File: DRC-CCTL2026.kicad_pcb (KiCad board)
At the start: 2 copper layers, 80 x 60 mm, 72 parts, among them J1 USB, J10 SW3, J12 LCD_BackLight, J2 FDCAN1, J3 FDCAN2, J4 FDCAN3, J5 SW1, J6 SW2, J7 STLINK, J8 I2C, J9 USART, Q1 MMBT3904, SW1 RESET, SW2 DIP, U1 STM32G474RETx, U2 AZ1084C-3.3, U3 74AHC1G125, Y1 8M10PB/XT324-10/80

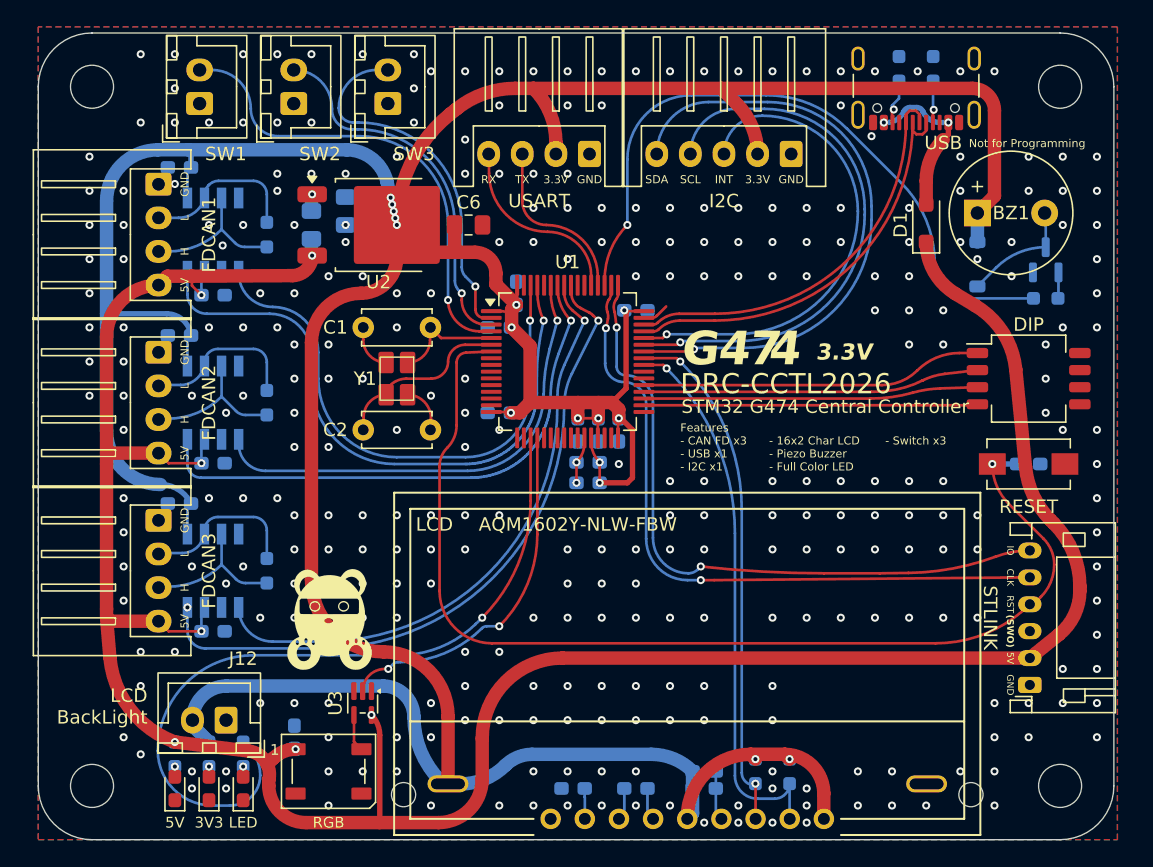
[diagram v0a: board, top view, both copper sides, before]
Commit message: v0.2.0
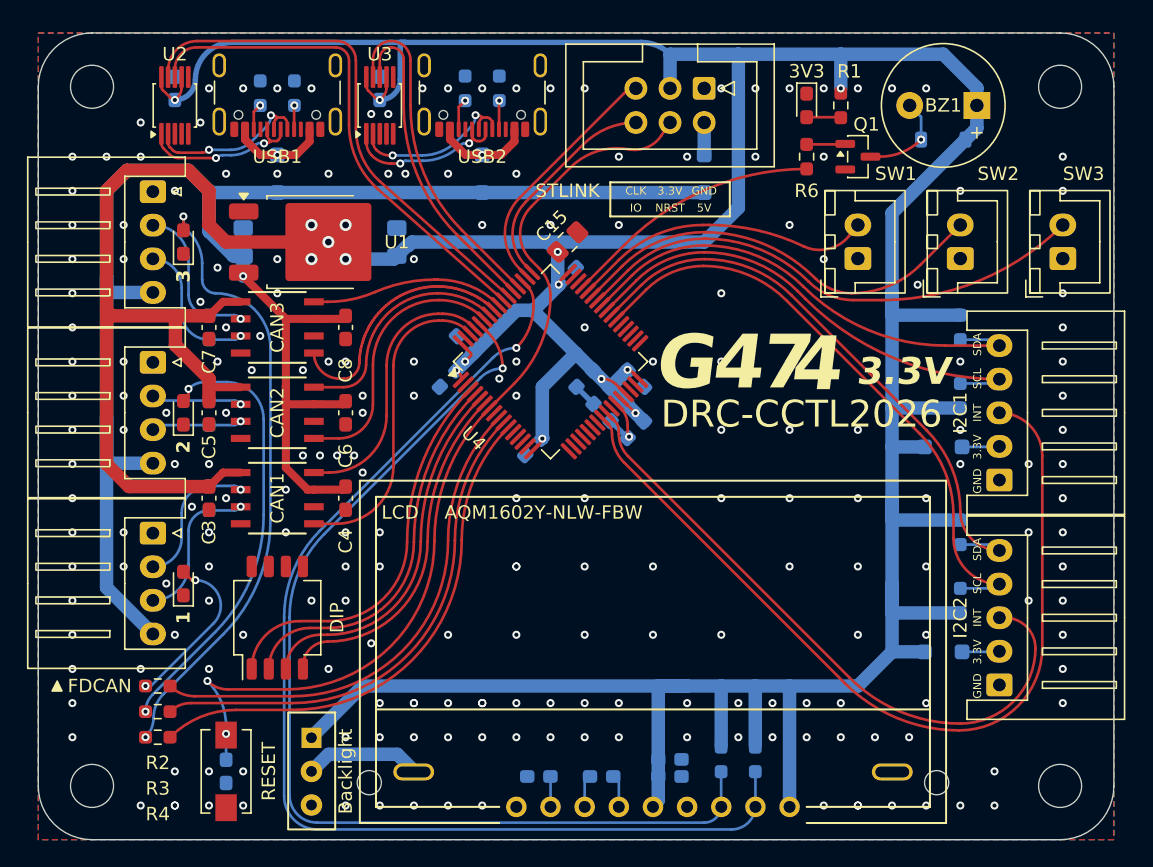
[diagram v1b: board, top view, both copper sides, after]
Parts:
- removed the C1 at (139.2, 91.9)
- removed the C10 at (145.6, 89.4)
- removed the C11 at (150.1, 99.5)
- removed the C12 at (151.7, 99.5)
- removed the C2 at (134.2, 99.5)
- removed the C3 at (183.7, 102.1)
- removed the C6 at (142.0, 84.3)
- removed the C7 at (144.3, 98.2)
- removed the C8 at (153.2, 99.5)
- removed the C9 at (154.4, 90.6)
- removed the D1 at (176.0, 84.2)
- removed the J1 at (175.3, 73.0)
- removed J12: LCD_BackLight, Connector_JST:JST_XH_B2B-XH-A_1x02_P2.50mm_Vertical
- removed the R1 at (176.6, 72.7)
- removed R5: 1k, Resistor_SMD:R_0603_1608Metric_Pad0.98x0.95mm_HandSolder
- removed the R6 at (125.2, 123.7)
- removed the SW1 at (183.7, 102.1)
- removed the U1 at (149.4, 94.4)
- removed Y1: 8M10PB/XT324-10/80, lib:8M10PB_XT324-10_80
- added C17: 0.1u, Capacitor_SMD:C_0603_1608Metric_Pad1.08x0.95mm_HandSolder, B.Cu at (154.4, 95.7)
- added C18: 0.1u, Capacitor_SMD:C_0603_1608Metric_Pad1.08x0.95mm_HandSolder, B.Cu at (149.4, 88.1)
- added C19: 0.1u, Capacitor_SMD:C_0603_1608Metric_Pad1.08x0.95mm_HandSolder, B.Cu at (141.8, 93.2)
- added C20: 1u, Capacitor_SMD:C_0603_1608Metric_Pad1.08x0.95mm_HandSolder, B.Cu at (150.6, 95.7)
- added C21: 0.1u, Capacitor_SMD:C_0603_1608Metric_Pad1.08x0.95mm_HandSolder, B.Cu at (151.9, 97.0)
- added C22: 1u, Capacitor_SMD:C_0603_1608Metric_Pad1.08x0.95mm_HandSolder, B.Cu at (154.4, 99.5)
- added C23: 0.1u, Capacitor_SMD:C_0603_1608Metric_Pad1.08x0.95mm_HandSolder, B.Cu at (153.2, 98.2)
- added C24: 1u, Capacitor_SMD:C_0603_1608Metric_Pad1.08x0.95mm_HandSolder, B.Cu at (140.5, 95.7)
- added C25: 0.1u, Capacitor_SMD:C_0603_1608Metric_Pad1.08x0.95mm_HandSolder, B.Cu at (124.0, 124.9)
- added D10: SS2040FL, Diode_SMD:D_SOD-123F, B.Cu at (127.8, 80.5)
- added D11: SS2040FL, Diode_SMD:D_SOD-123F, B.Cu at (143.0, 80.5)
- added D3: SS2040FL, Diode_SMD:D_SOD-123F, B.Cu at (177.3, 100.8)
- added D7: LED2, LED_SMD:LED_0603_1608Metric_Pad1.05x0.95mm_HandSolder, F.Cu at (120.8, 98.2)
- added D8: LED3, LED_SMD:LED_0603_1608Metric_Pad1.05x0.95mm_HandSolder, F.Cu at (120.8, 85.5)
- added J10: USB_C, Connector_USB:USB_C_Receptacle_GCT_USB4105-xx-A_16P_TopMnt_Horizontal, F.Cu at (127.8, 73.5)
- added J11: USB_C, Connector_USB:USB_C_Receptacle_GCT_USB4105-xx-A_16P_TopMnt_Horizontal, F.Cu at (143.0, 73.5)
- added R12: 5.1k, Resistor_SMD:R_0603_1608Metric_Pad0.98x0.95mm_HandSolder, B.Cu at (129.1, 74.5)
- added R13: 5.1k, Resistor_SMD:R_0603_1608Metric_Pad0.98x0.95mm_HandSolder, B.Cu at (126.5, 74.5)
- added R14: 5.1k, Resistor_SMD:R_0603_1608Metric_Pad0.98x0.95mm_HandSolder, B.Cu at (144.3, 74.1)
- added R15: 5.1k, Resistor_SMD:R_0603_1608Metric_Pad0.98x0.95mm_HandSolder, B.Cu at (141.8, 74.1)
- added R16: 4.7k, Resistor_SMD:R_0603_1608Metric_Pad0.98x0.95mm_HandSolder, B.Cu at (178.6, 91.9)
- added R17: 4.7k, Resistor_SMD:R_0603_1608Metric_Pad0.98x0.95mm_HandSolder, B.Cu at (178.6, 97.0)
- added R18: 4.7k, Resistor_SMD:R_0603_1608Metric_Pad0.98x0.95mm_HandSolder, B.Cu at (178.6, 107.1)
- added R19: 4.7k, Resistor_SMD:R_0603_1608Metric_Pad0.98x0.95mm_HandSolder, B.Cu at (178.6, 112.2)
- added R3: 1k, Resistor_SMD:R_0603_1608Metric_Pad0.98x0.95mm_HandSolder, F.Cu at (118.9, 120.5)
- added R4: 1k, Resistor_SMD:R_0603_1608Metric_Pad0.98x0.95mm_HandSolder, F.Cu at (118.9, 122.4)
- added SW2: SS-12D00G3, lib:SS-12D00G3, F.Cu at (130.3, 124.9)
- added SW3: SW_Push, Button_Switch_SMD:SW_SPST_EVQPE1, F.Cu at (124.0, 124.9)
- added U2: CH340E, Package_SO:MSOP-10_3x3mm_P0.5mm, F.Cu at (120.2, 75.4)
- added U4: STM32G474RETx, Package_QFP:LQFP-64_10x10mm_P0.5mm, F.Cu at (148.1, 94.4)
- C13, C16: value 1u -> 0.1u
- C15: value 0.1u -> 4.7u; footprint Capacitor_SMD:C_0603_1608Metric_Pad1.08x0.95mm_HandSolder -> Capacitor_SMD:C_0805_2012Metric_Pad1.18x1.45mm_HandSolder; moved to F.Cu
- C3: renamed from C17; moved to F.Cu
- C4: renamed from C18; moved to F.Cu
- C5: renamed from C19; moved to F.Cu
- C6: renamed from C20; moved to F.Cu
- C7: renamed from C21; moved to F.Cu
- C8: renamed from C22; moved to F.Cu
- CAN1: renamed from FDCAN1; footprint footprints:SOIC127P600X175-8N -> lib:SO8_SOT96-1_NXP; moved to F.Cu
- CAN2: renamed from FDCAN2; footprint footprints:SOIC127P600X175-8N -> lib:SO8_SOT96-1_NXP; moved to F.Cu
- CAN3: renamed from FDCAN3; footprint footprints:SOIC127P600X175-8N -> lib:SO8_SOT96-1_NXP; moved to F.Cu
- D2: value 1N4148W -> SS2040FL; footprint Diode_SMD:D_SOD-123 -> Diode_SMD:D_SOD-123F
- D4: value RGB -> SS2040FL; footprint LED_SMD:LED_WS2812B_PLCC4_5.0x5.0mm_P3.2mm -> Diode_SMD:D_SOD-123F; moved to B.Cu
- D5: value 5V -> 1N4148W; footprint LED_SMD:LED_0603_1608Metric_Pad1.05x0.95mm_HandSolder -> Diode_SMD:D_SOD-123; moved to B.Cu
- D6: value LED -> LED1
- G***: moved to B.Cu
- J1: renamed from J7; footprint Connector_JST:JST_PH_S6B-PH-K_1x06_P2.00mm_Horizontal -> Connector_IDC:IDC-Header_2x03_P2.54mm_Vertical
- J8: value I2C -> I2C1
- J9: value USART -> I2C2; footprint Connector_JST:JST_XH_S4B-XH-A_1x04_P2.50mm_Horizontal -> Connector_JST:JST_XH_S5B-XH-A_1x05_P2.50mm_Horizontal
- Q1: moved to F.Cu
- R1: renamed from R4; value 470 -> 1k; moved to F.Cu
- R2: value 5.1k -> 1k; moved to F.Cu
- R6: renamed from R3; moved to F.Cu
- U3: value 74AHC1G125 -> CH340E; footprint Package_TO_SOT_SMD:SOT-353_SC-70-5 -> Package_SO:MSOP-10_3x3mm_P0.5mm
- moved D5 74.8 mm to (177.3, 77.9), turned to 180 degrees
- moved R2 71.7 mm to (118.9, 118.6), turned to 180 degrees
- moved D1 67.5 mm to (167.2, 75.4), turned to -90 degrees
- moved R1 67.4 mm to (169.7, 75.4)
- moved SW1 58.6 mm to (127.8, 113.5), turned to 90 degrees
- moved J7 51.5 mm to (186.2, 86.8)
- moved J6 50.9 mm to (178.6, 86.8)
- moved J1 50.6 mm to (159.5, 74.1), turned to -90 degrees
- moved J5 50.3 mm to (171.0, 86.8)
- moved J9 49.9 mm to (181.5, 118.5), turned to 90 degrees
- moved C14 49.1 mm to (120.2, 74.1)
- moved D4 46.6 mm to (177.3, 116.0), turned to 180 degrees
- moved U3 44.5 mm to (135.4, 75.4), turned to 90 degrees
- moved G*** 34.0 mm to (165.3, 108.5), turned to 180 degrees
- moved C13 31.8 mm to (135.4, 74.1), turned to -90 degrees
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- renumbered C4 to C1, C24 to C10, C25 to C11, C26 to C12, C5 to C2, C23 to C9, D3 to D1, J10 to J7, SW2 to SW1, U2 to U1
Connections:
- net /LCD_SCL renamed /LCD/LCD_SCL
- net /LCD_SDA renamed /LCD/LCD_SDA
- C13 pad 1: +3V3 -> GND
- C13 pad 2: GND -> +3V3
- C14 pad 2: +5V -> +3V3
- CAN1 pad 1: /FDCAN1_TX -> /FDCAN1/FDCAN_TX
- CAN1 pad 4: /FDCAN1_RX -> /FDCAN1/FDCAN_RX
- CAN2 pad 1: /FDCAN2_TX -> /FDCAN2/FDCAN_TX
- CAN2 pad 4: /FDCAN2_RX -> /FDCAN2/FDCAN_RX
- CAN3 pad 1: /FDCAN3_TX -> /FDCAN3/FDCAN_TX
- CAN3 pad 4: /FDCAN3_RX -> /FDCAN3/FDCAN_RX
- D2 pad 1: +3V3 -> +5V
- D2 pad 2: Net-(BZ1--) -> Net-(D2-A)
- D4 pad 1: +5V -> Net-(D4-K)
- D4 pad 2: unconnected-(D4-DOUT-Pad2) -> +3V3
- D5 pad 1: GND -> +3V3
- D5 pad 2: Net-(D5-A) -> Net-(BZ1--)
- J1 pad 2: +5V -> Net-(D2-A)
- J1 pad 3: unconnected-(J7-Pin_3-Pad3) -> +3V3
- J5 pad 2: /SW1 -> /STM32G474/SW1
- J6 pad 2: /SW2 -> /STM32G474/SW2
- J7 pad 2: /SW3 -> /STM32G474/SW3
- J8 pad 2: +3V3 -> Net-(D3-K)
- J8 pad 3: /I2C_INT -> /STM32G474/I2C1_INT
- J8 pad 4: /I2C_SCL -> /STM32G474/I2C1_SCL
- J8 pad 5: /I2C_SDA -> /STM32G474/I2C1_SDA
- J9 pad 2: +3V3 -> Net-(D4-K)
- J9 pad 3: /USART_TX -> /STM32G474/I2C2_INT
- J9 pad 4: /USART_RX -> /STM32G474/I2C2_SCL
- LCD1 pad A: +3V3 -> Net-(SW2-B)
- R2 pad 1: Net-(J1-CC2) -> /STM32G474/LED1
- R2 pad 2: GND -> Net-(D6-A)
- R6 pad 1: /BUZZER -> /STM32G474/BZ_TIM1_CH4
- SW1 pad 1: /DIP1 -> /STM32G474/DIP1
- SW1 pad 2: /DIP2 -> /STM32G474/DIP2
- SW1 pad 3: /DIP3 -> /STM32G474/DIP3
- SW1 pad 4: /DIP4 -> /STM32G474/DIP4
- U3 pad 1: GND -> /USBC2/USB_D_P
- U3 pad 2: /RGB -> /USBC2/USB_D_N
- U3 pad 4: Net-(D4-DIN) -> unconnected-(U3-~{RTS}-Pad4)
- U3 pad 5: +5V -> unconnected-(U3-~{CTS}-Pad5)
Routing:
- net +3V3: track 325.8 -> 402.9 mm, vias 17 -> 16
- net /STM32G474/I2C1_INT: track 0.00 -> 65.0 mm
- net +5V: track 195.5 -> 130.8 mm, vias 7 -> 1
- net /LED_BI: track 56.8 -> 0.00 mm, vias 1 -> 0
- net /FDCAN3_RX: track 50.5 -> 0.00 mm, vias 2 -> 0
- net /BUZZER: track 50.3 -> 0.00 mm, vias 1 -> 0
- net /STM32G474/I2C2_INT: track 0.00 -> 48.5 mm
- net /FDCAN1_RX: track 46.4 -> 0.00 mm, vias 1 -> 0
- net Net-(D8-A): track 0.00 -> 45.9 mm, vias 0 -> 2
- net /STM32G474/I2C2_SCL: track 0.00 -> 45.3 mm
- net /I2C_SDA: track 45.3 -> 0.00 mm, vias 1 -> 0
- net /LCD/LCD_SCL: track 41.6 -> 86.0 mm
- net /FDCAN3_TX: track 44.4 -> 0.00 mm, vias 1 -> 0
- net /STM32G474/I2C2_SDA: track 0.00 -> 43.9 mm
- net /FDCAN2_RX: track 41.6 -> 0.00 mm, vias 1 -> 0
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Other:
- board text added: "1"
- board text added: "2"
- board text added: "3"
- board text added: "DRC-CCTL2026 v0.2.0"
- board text added: "Designed by kotek, March 2026"
- board text added: "FDCAN"
- board text added: "NRST"
- board text removed: "(SWO)"
- board text removed: "- 16x2 Char LCD - Piezo Buzzer - Full Color LED"
- board text removed: "- CAN FD x3 - USB x1 - I2C x1"
- board text removed: "- Switch x3"
- board text removed: "Created by kotek, March 2026"
- board text removed: "DRC-CCTL2026 v0.1.0"
- board text removed: "Features"
- board text removed: "LCD BackLight"
- board text removed: "Not for Programming"
- board text removed: "RST"
- board text removed: "RX"
- board text removed: "TX"
